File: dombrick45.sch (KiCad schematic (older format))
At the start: 114 parts, among them SW1 SW_Push, U1 ATmega32U4-AU, Y1 16MHz

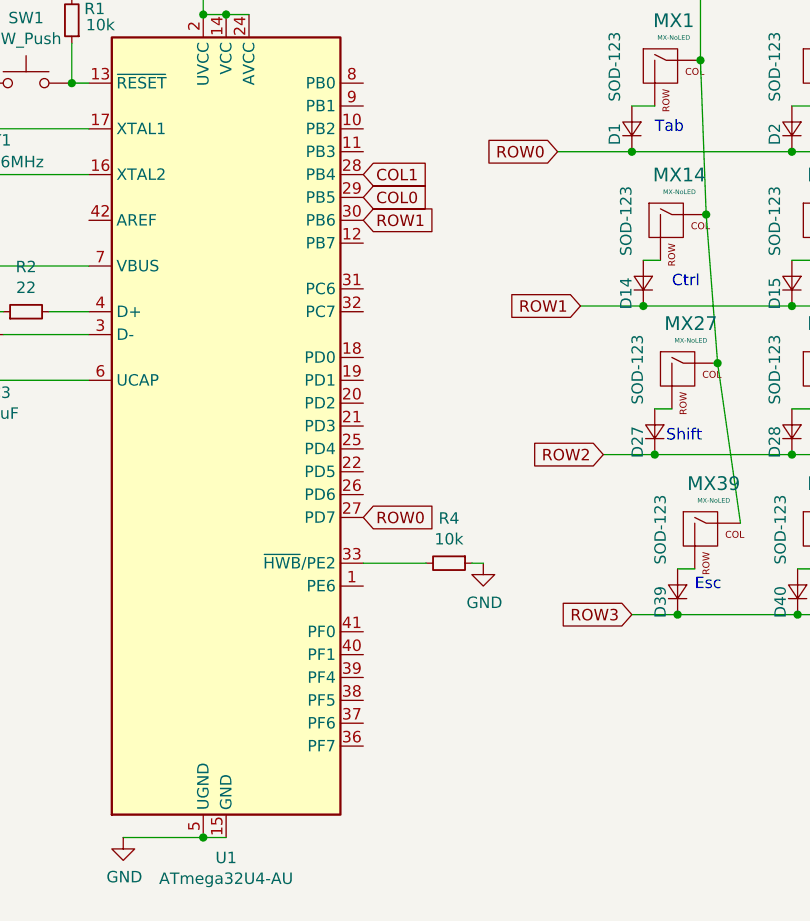
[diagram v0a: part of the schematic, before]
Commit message: 2019-10-12 PBC ver0.1
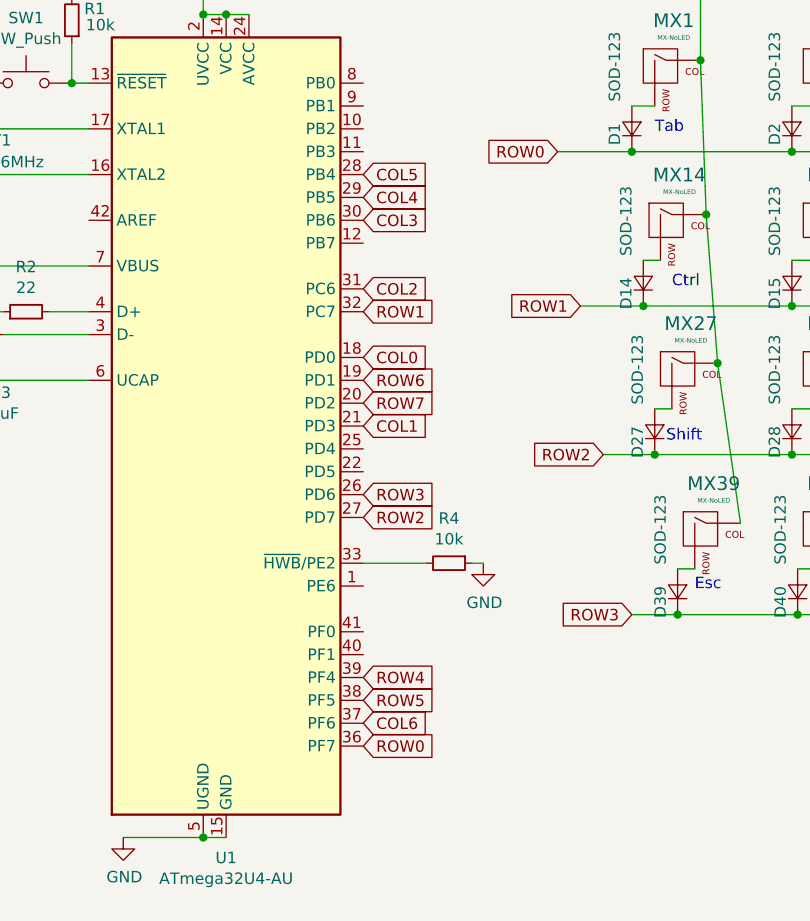
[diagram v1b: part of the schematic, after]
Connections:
- net COL0: now also U1.18 (PD0); no longer U1.29 (PB5)
- net COL1: now also U1.21 (PD3); no longer U1.28 (PB4)
- net COL2: now also U1.31 (PC6)
- net COL3: now also U1.30 (PB6)
- net COL4: now also U1.29 (PB5)
- net COL5: now also U1.28 (PB4)
- net COL6: now also U1.37 (PF6)
- net ROW0: now also U1.36 (PF7); no longer U1.27 (PD7)
- net ROW1: now also U1.32 (PC7); no longer U1.30 (PB6)
- net ROW2: now also U1.27 (PD7)
- net ROW3: now also U1.26 (PD6)
- net ROW4: now also U1.39 (PF4)
- net ROW5: now also U1.38 (PF5)
- net ROW6: now also U1.19 (PD1)
- net ROW7: now also U1.20 (PD2)
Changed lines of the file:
@@
 Text GLabel 3875 2325 0    50   Input ~ 0
 ROW1
-Text GLabel 2925 3250 2    50   Input ~ 0
-ROW0
-Text GLabel 2925 1950 2    50   Input ~ 0
-ROW1
-Text GLabel 2925 1850 2    50   Input ~ 0
-COL0
-Text GLabel 2925 1750 2    50   Input ~ 0
-COL1
 NoConn ~ 2125 6200
 Text GLabel 875  2450 0    50   Input ~ 0
@@
 Wire Wire Line
 	9200 3675 9650 3675
+Text GLabel 2925 4250 2    50   Input ~ 0
+ROW0
+Text GLabel 2925 4150 2    50   Input ~ 0
+COL6
+Text GLabel 2925 4050 2    50   Input ~ 0
+ROW5
+Text GLabel 2925 3950 2    50   Input ~ 0
+ROW4
+Text GLabel 2925 2350 2    50   Input ~ 0
+ROW1
+Text GLabel 2925 2250 2    50   Input ~ 0
+COL2
+Text GLabel 2925 1950 2    50   Input ~ 0
+COL3
+Text GLabel 2925 1850 2    50   Input ~ 0
+COL4
+Text GLabel 2925 1750 2    50   Input ~ 0
+COL5
+Text GLabel 2925 3250 2    50   Input ~ 0
+ROW2
+Text GLabel 2925 3150 2    50   Input ~ 0
+ROW3
+Text GLabel 2925 2850 2    50   Input ~ 0
+COL1
+Text GLabel 2925 2750 2    50   Input ~ 0
+ROW7
+Text GLabel 2925 2650 2    50   Input ~ 0
+ROW6
+Text GLabel 2925 2550 2    50   Input ~ 0
+COL0
 $EndSCHEMATC
